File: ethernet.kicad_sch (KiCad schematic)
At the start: 32 parts, among them J5 1888250-3, U3 W5500, X1 25MHz

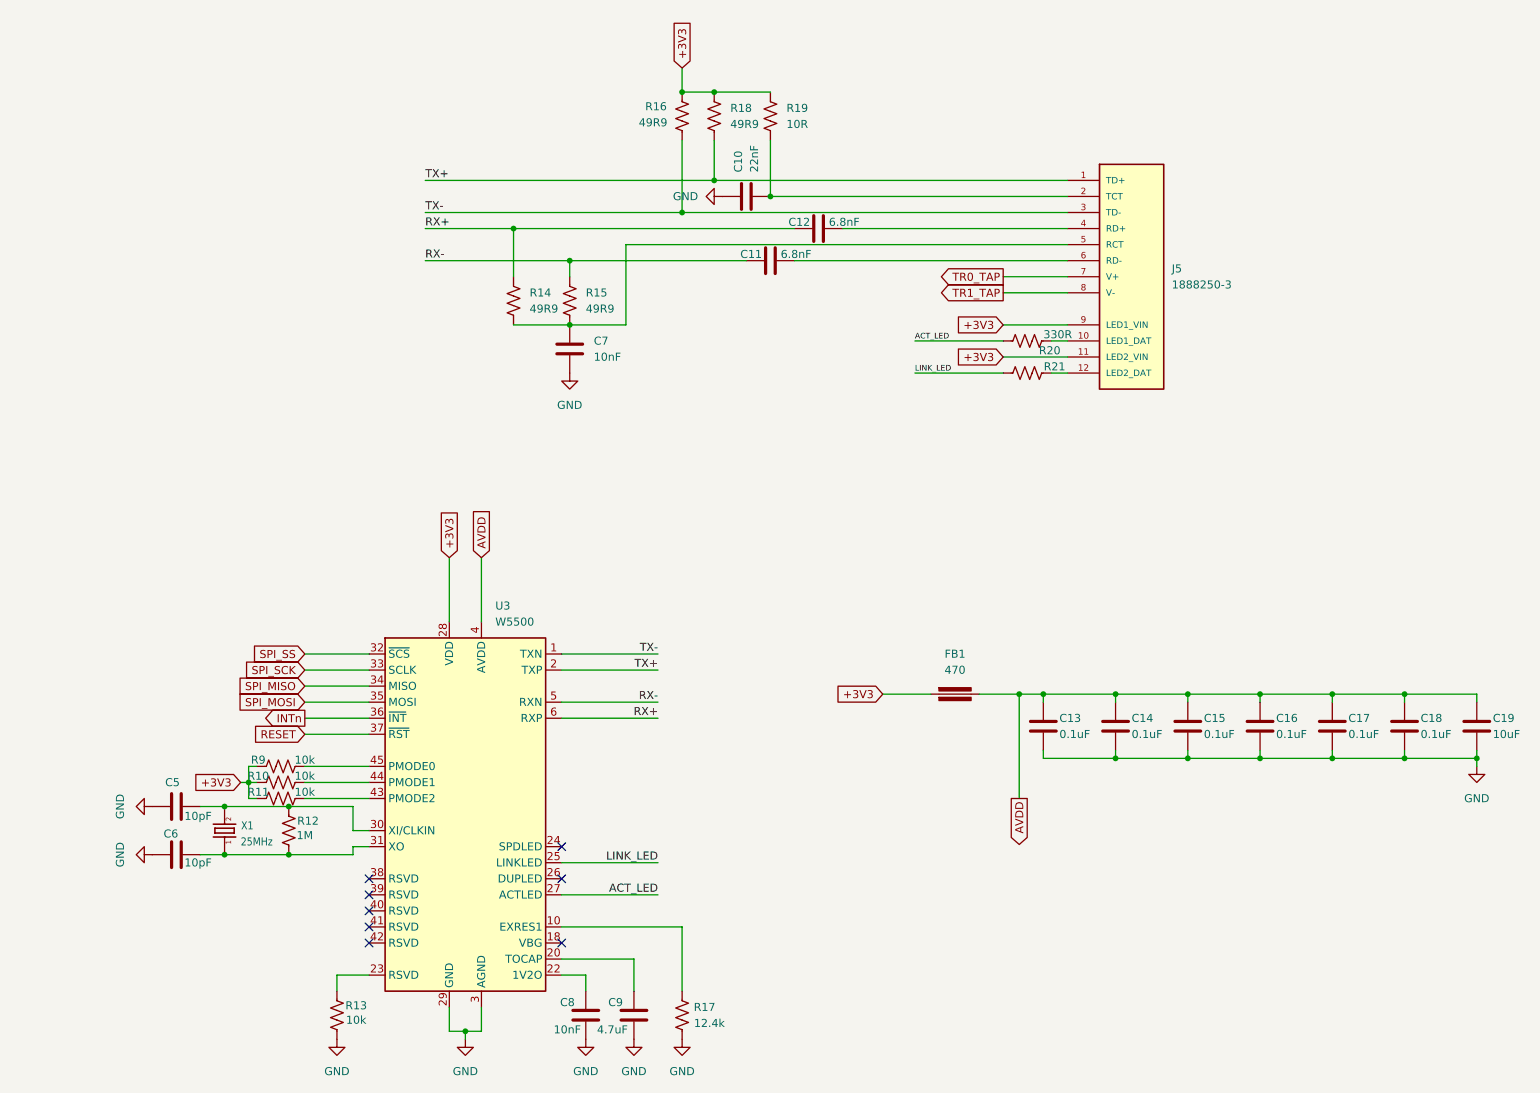
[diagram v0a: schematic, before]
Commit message: Recent updates
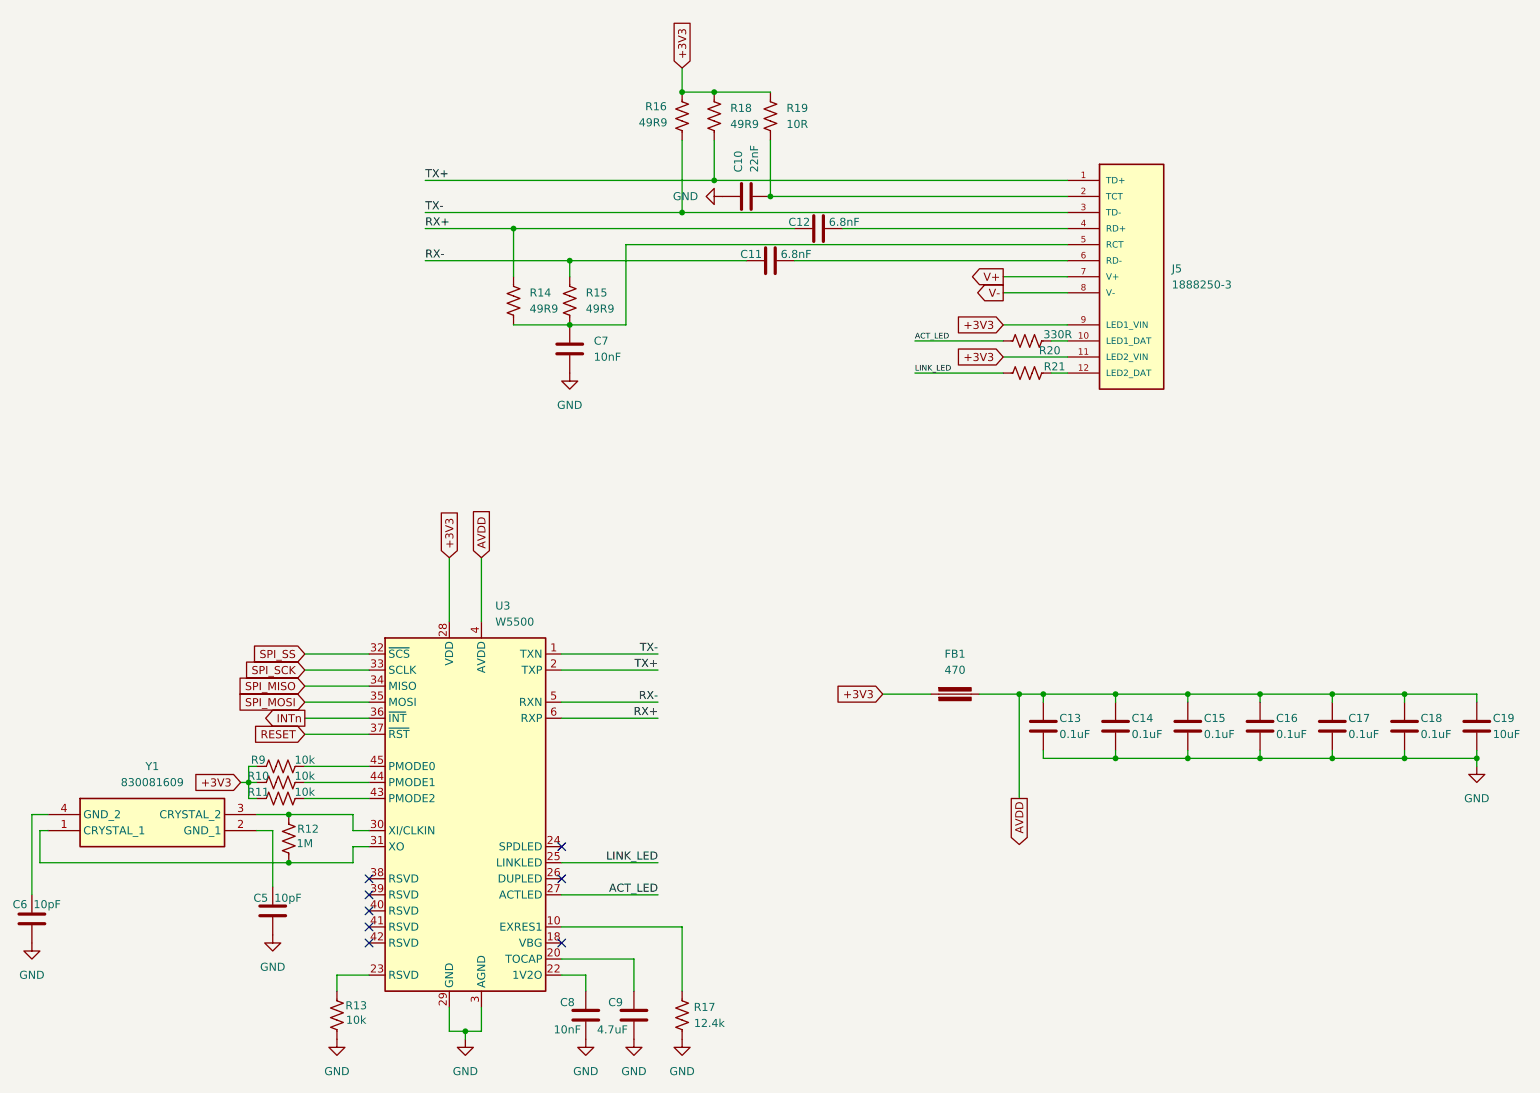
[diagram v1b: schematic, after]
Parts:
- removed X1: 25MHz, Crystal:Crystal_SMD_TXC_9HT11-2Pin_2.0x1.2mm_HandSoldering, symbol seeed-eagle-import:CRYSTAL'5032'
- added Y1: 830081609, CrystalOscillator:830081609, symbol CrystalOscillator:830081609
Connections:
- net at R12.2, U3.30 (XI/CLKIN): now also Y1.3 (CRYSTAL_2); no longer C5.1
- net at R12.1, U3.31 (XO): now also Y1.1 (CRYSTAL_1); no longer C6.1
- net TR0_TAP renamed V+
- net TR1_TAP renamed V-
- new net: C5.1, Y1.2 (GND_1)
- new net: C6.1, Y1.4 (GND_2)
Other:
- moved on the sheet: C5, C6, R12
